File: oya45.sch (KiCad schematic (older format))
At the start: 94 parts, among them U1 ProMicro

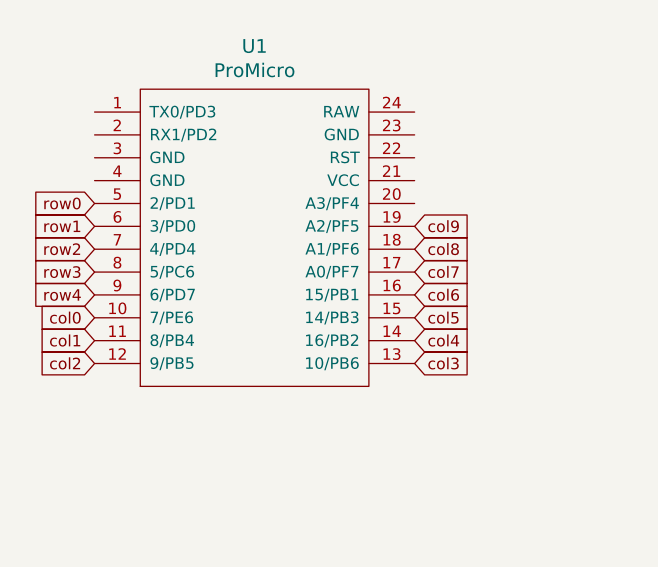
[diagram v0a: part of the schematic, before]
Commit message: pro micro first clean routing
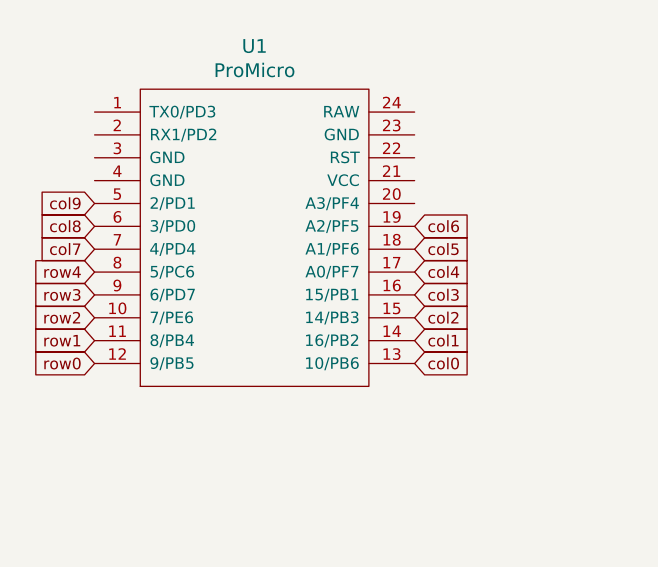
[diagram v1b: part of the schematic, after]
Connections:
- net col0: now also U1.13 (10/PB6); no longer U1.10 (7/PE6)
- net col1: now also U1.14 (16/PB2); no longer U1.11 (8/PB4)
- net col2: now also U1.15 (14/PB3); no longer U1.12 (9/PB5)
- net col3: now also U1.16 (15/PB1); no longer U1.13 (10/PB6)
- net col4: now also U1.17 (A0/PF7); no longer U1.14 (16/PB2)
- net col5: now also U1.18 (A1/PF6); no longer U1.15 (14/PB3)
- net col6: now also U1.19 (A2/PF5); no longer U1.16 (15/PB1)
- net col7: now also U1.7 (4/PD4); no longer U1.17 (A0/PF7)
- net col8: now also U1.6 (3/PD0); no longer U1.18 (A1/PF6)
- net col9: now also U1.5 (2/PD1); no longer U1.19 (A2/PF5)
- net row0: now also U1.12 (9/PB5); no longer U1.5 (2/PD1)
- net row1: now also U1.11 (8/PB4); no longer U1.6 (3/PD0)
- net row2: now also U1.10 (7/PE6); no longer U1.7 (4/PD4)
- net row3: now also U1.9 (6/PD7); no longer U1.8 (5/PC6)
- net row4: now also U1.8 (5/PC6); no longer U1.9 (6/PD7)
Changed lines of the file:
@@
 Text GLabel 5250 5200 0    50   Input ~ 0
 row4
+Text GLabel 3700 3400 2    50   Input ~ 0
+col3
+Text GLabel 3700 3300 2    50   Input ~ 0
+col4
+Text GLabel 3700 3200 2    50   Input ~ 0
+col5
+Text GLabel 3700 3100 2    50   Input ~ 0
+col6
+Text GLabel 2300 3200 0    50   Input ~ 0
+col7
+Text GLabel 2300 3100 0    50   Input ~ 0
+col8
 Text GLabel 2300 3000 0    50   Input ~ 0
-row0
-Text GLabel 2300 3100 0    50   Input ~ 0
-row1
-Text GLabel 2300 3200 0    50   Input ~ 0
-row2
-Text GLabel 2300 3300 0    50   Input ~ 0
-row3
-Text GLabel 2300 3400 0    50   Input ~ 0
-row4
-Text GLabel 2300 3500 0    50   Input ~ 0
-col0
-Text GLabel 2300 3600 0    50   Input ~ 0
-col1
-Text GLabel 2300 3700 0    50   Input ~ 0
-col2
-Text GLabel 3700 3700 2    50   Input ~ 0
-col3
-Text GLabel 3700 3600 2    50   Input ~ 0
-col4
-Text GLabel 3700 3500 2    50   Input ~ 0
-col5
-Text GLabel 3700 3400 2    50   Input ~ 0
-col6
-Text GLabel 3700 3300 2    50   Input ~ 0
-col7
-Text GLabel 3700 3200 2    50   Input ~ 0
-col8
-Text GLabel 3700 3100 2    50   Input ~ 0
 col9
 Connection ~ 5750 1800
@@
 	1    0    0    -1
 $EndComp
+Text GLabel 2300 3700 0    50   Input ~ 0
+row0
+Text GLabel 2300 3600 0    50   Input ~ 0
+row1
+Text GLabel 2300 3500 0    50   Input ~ 0
+row2
+Text GLabel 2300 3400 0    50   Input ~ 0
+row3
+Text GLabel 2300 3300 0    50   Input ~ 0
+row4
+Text GLabel 3700 3700 2    50   Input ~ 0
+col0
+Text GLabel 3700 3600 2    50   Input ~ 0
+col1
+Text GLabel 3700 3500 2    50   Input ~ 0
+col2
 $EndSCHEMATC
